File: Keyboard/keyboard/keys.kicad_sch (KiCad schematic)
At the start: 26 parts, among them SW10 Cherry_MX_1u, SW11 Cherry_MX_1u, SW12 Cherry_MX_1u, SW13 Cherry_MX_1u, SW2 Cherry_MX_1u, SW3 Cherry_MX_1u, SW4 Cherry_MX_1u, SW5 Cherry_MX_1u, SW6 Cherry_MX_1u, SW7 Cherry_MX_1u, SW8 Cherry_MX_1u, SW9 Cherry_MX_1u

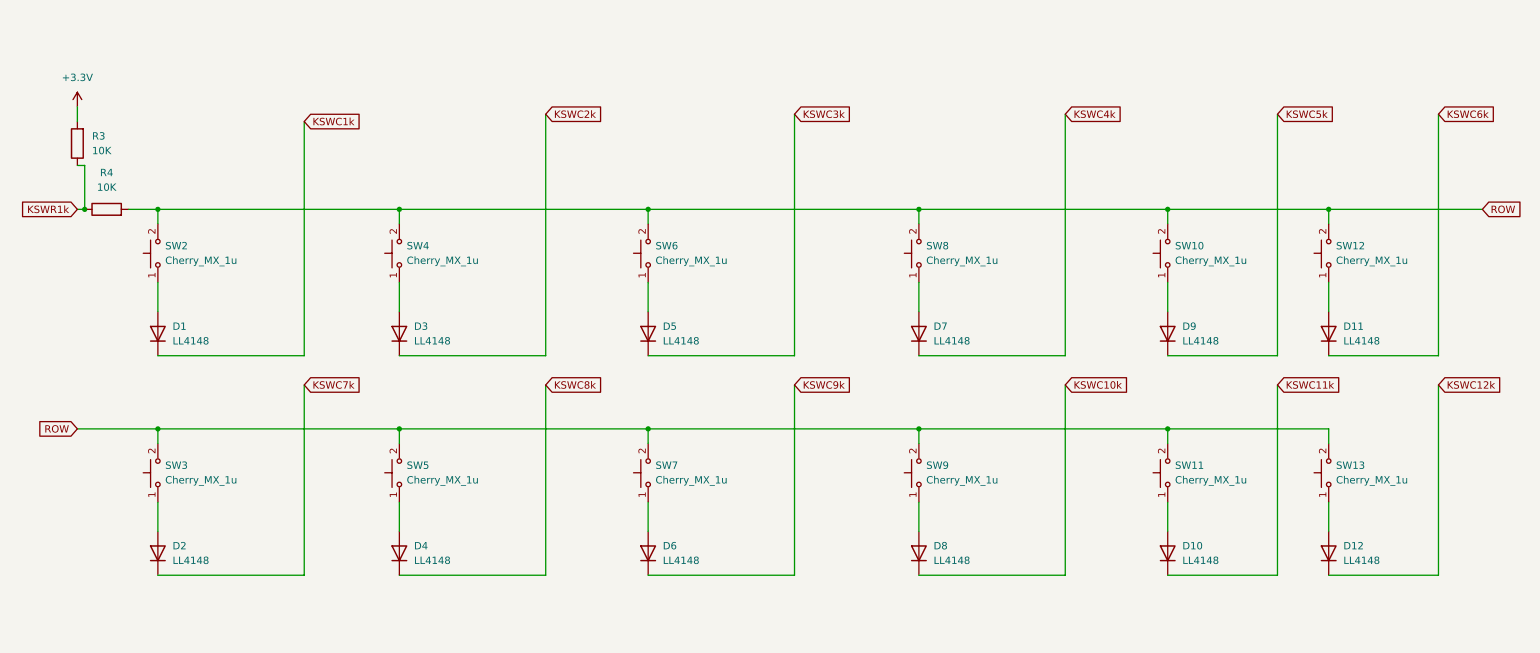
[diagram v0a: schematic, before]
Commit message: pcb design fixing
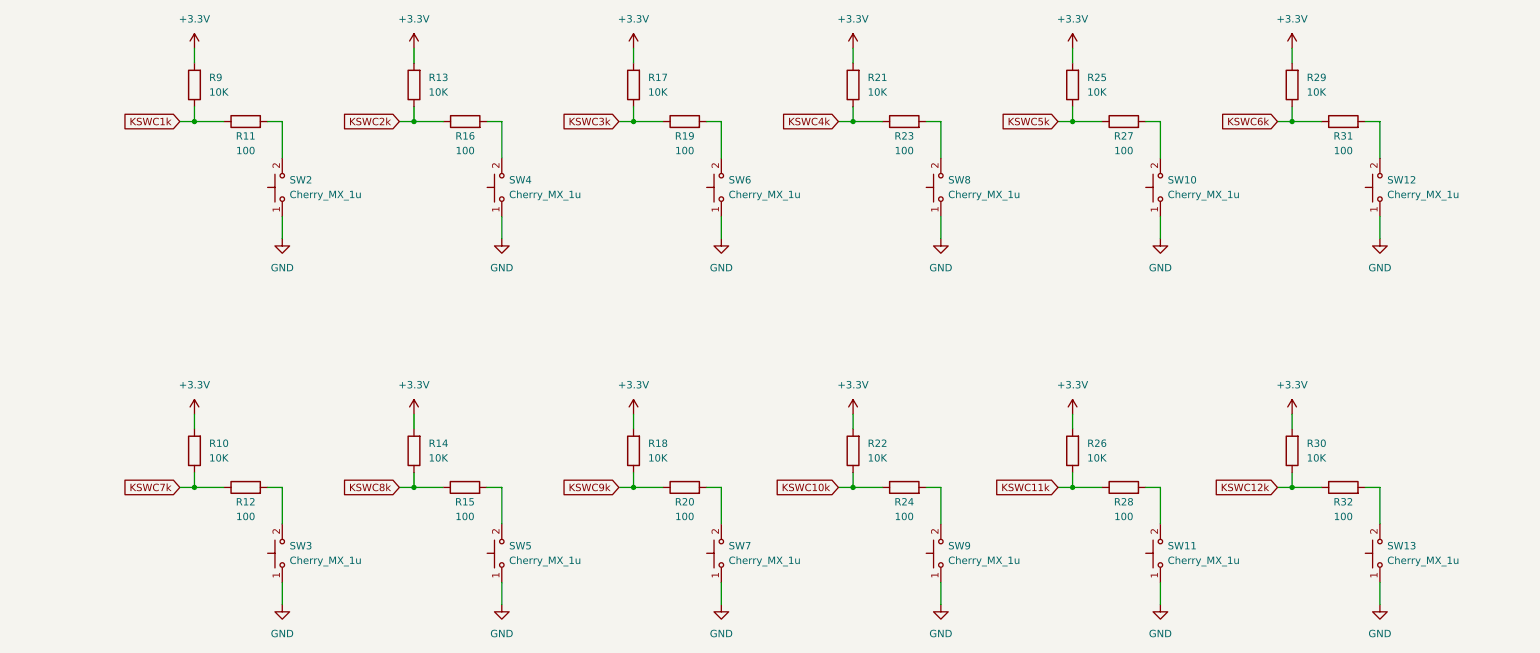
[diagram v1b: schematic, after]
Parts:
- removed D1, D10, D11, D12, D2, D3, D4, D5, D6, D7, D8, D9: LL4148, Diode_SMD:D_MiniMELF, symbol Diode:LL4148
- removed R3, R4: 10K, Resistor_SMD:R_0805_2012Metric_Pad1.20x1.40mm_HandSolder, symbol Device:R
- added R10, R13, R14, R17, R18, R21, R22, R25, R26, R29, R30, R9: 10K, Resistor_SMD:R_0805_2012Metric_Pad1.20x1.40mm_HandSolder, symbol Device:R
- added R11, R12, R15, R16, R19, R20, R23, R24, R27, R28, R31, R32: 100, Resistor_SMD:R_0805_2012Metric_Pad1.20x1.40mm_HandSolder, symbol Device:R
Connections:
- net +3V3: now also R10.2, R13.2, R14.2, R17.2, R18.2, R21.2, R22.2, R25.2, R26.2, R29.2, R30.2, R9.2
- net KSWC10k: now also R22.1, R24.1
- net KSWC11k: now also R26.1, R28.1
- net KSWC12k: now also R30.1, R32.1
- net KSWC1k: now also R11.1, R9.1
- net KSWC2k: now also R13.1, R16.1
- net KSWC3k: now also R17.1, R19.1
- net KSWC4k: now also R21.1, R23.1
- net KSWC5k: now also R25.1, R27.1
- net KSWC6k: now also R29.1, R31.1
- net KSWC7k: now also R10.1, R12.1
- net KSWC8k: now also R14.1, R15.1
- net KSWC9k: now also R18.1, R20.1
- net GND: now reaches SW9.1
- net GND: now also SW10.1, SW11.1, SW12.1, SW13.1, SW2.1, SW3.1, SW4.1, SW5.1, SW6.1, SW7.1, SW8.1
- removed net ROW: SW10.2, SW11.2, SW12.2, SW13.2, SW2.2, SW3.2, SW4.2, SW5.2, SW6.2, SW7.2, SW8.2, SW9.2
- new net: R32.2, SW13.2
- new net: R16.2, SW4.2
- new net: R19.2, SW6.2
- new net: R11.2, SW2.2
- new net: R27.2, SW10.2
- new net: R12.2, SW3.2
- new net: R31.2, SW12.2
- new net: R20.2, SW7.2
- new net: R23.2, SW8.2
- new net: R15.2, SW5.2
- new net: R24.2, SW9.2
- new net: R28.2, SW11.2
